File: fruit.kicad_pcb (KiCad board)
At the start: 2 copper layers, 161.6 x 100 mm, 178 parts, among them J1 PCB_Edge_PCI_Express_x4_Salmo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, J2 2086581051, J3 TSM-102-01-L-SV, J4 TSM-102-01-L-SV, J5 MEM2067-02-180-00-A_REVB, J6 USB4110-GF-A, J7 USB4110-GF-A, J8 1-2199119-6, U1 INA260, U10 LM3525M-H_NPOB, U11 USB3740B-AI2, U12 AP22653FDZ-7, U13 AP64501SP-13, U14 AP64501SP-13, U2 PCA9671BS,118, U3 PCA9671BS,118, U4 AP22653FDZ-7, U5 TPD8S009DSMR, U6 INA260, U7 MCP9808T-E_MC, U8 ADS7142IRUGR, U9 MCP9808T-E_MC

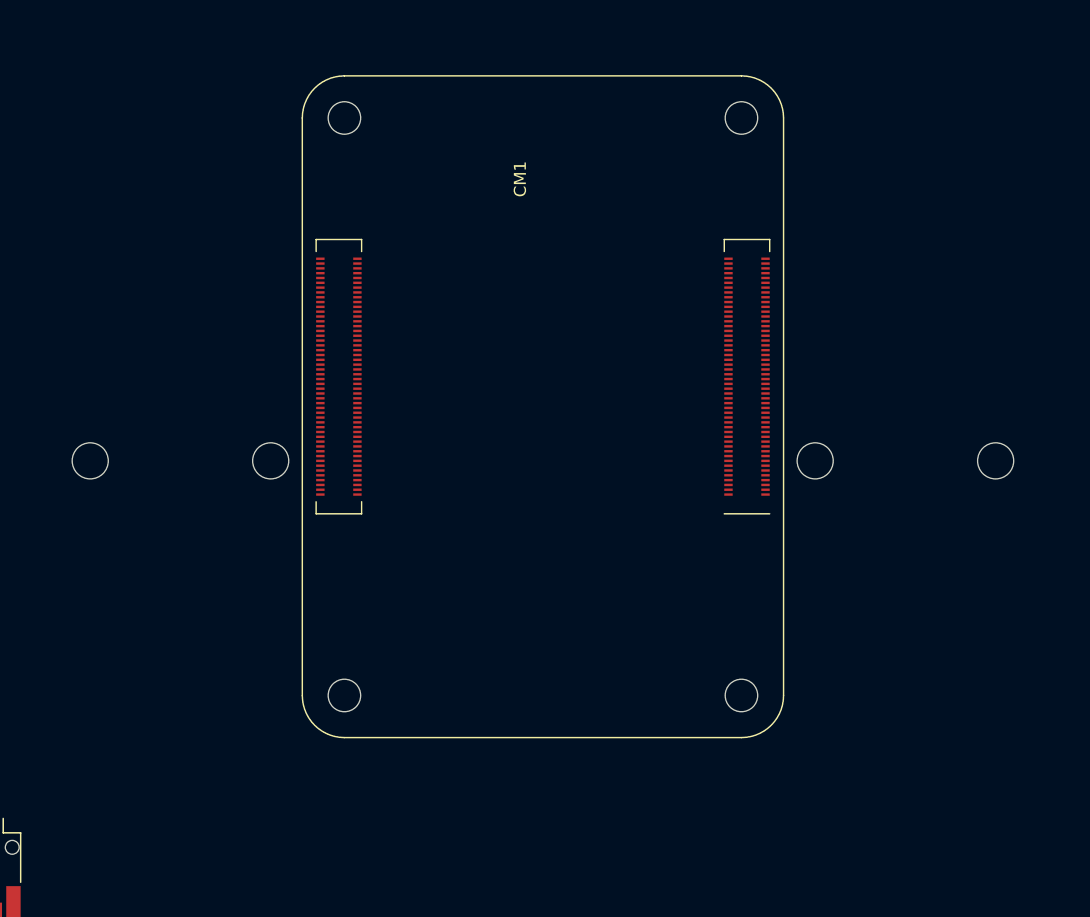
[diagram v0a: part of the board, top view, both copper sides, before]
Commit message: respin
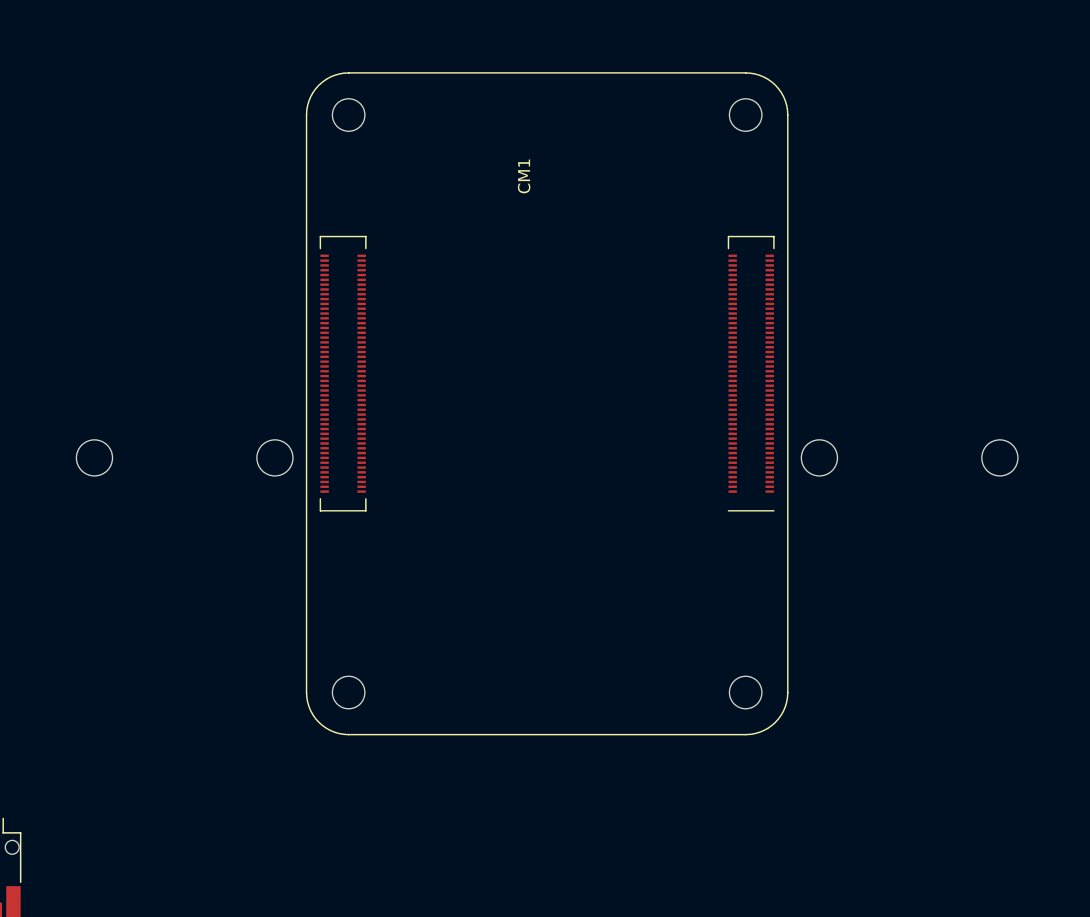
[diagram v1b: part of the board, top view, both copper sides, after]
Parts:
- moved CM1 0.43 mm to (121.4, 22.6)
- moved COOLER1 0.43 mm to (104.9, 51.1)
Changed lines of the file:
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@@
   )
   (footprint "Connector_RaspberryPi:Raspberry-Pi-4-Compute-Module_outline" (layer "F.Cu")
-    (at 121.05 22.86 180)
+    (at 121.402 22.614 180)
     (descr "Raspberry Pi 4 Compute Module")
     (tags "Raspberry Pi 4 Compute Module")
@@
   )
   (footprint "Mechanical_CoolingBlock:53-61mm_NorthBridge_45deg_arms" (layer "F.Cu")
-    (at 104.55 51.3 90)
+    (at 104.902 51.054 90)
     (descr "53-61mm mounting hole pattern and NorthBridge, 45 deg offset, and arms -- combined.")
     (property "Sheetfile" "fruit.kicad_sch")

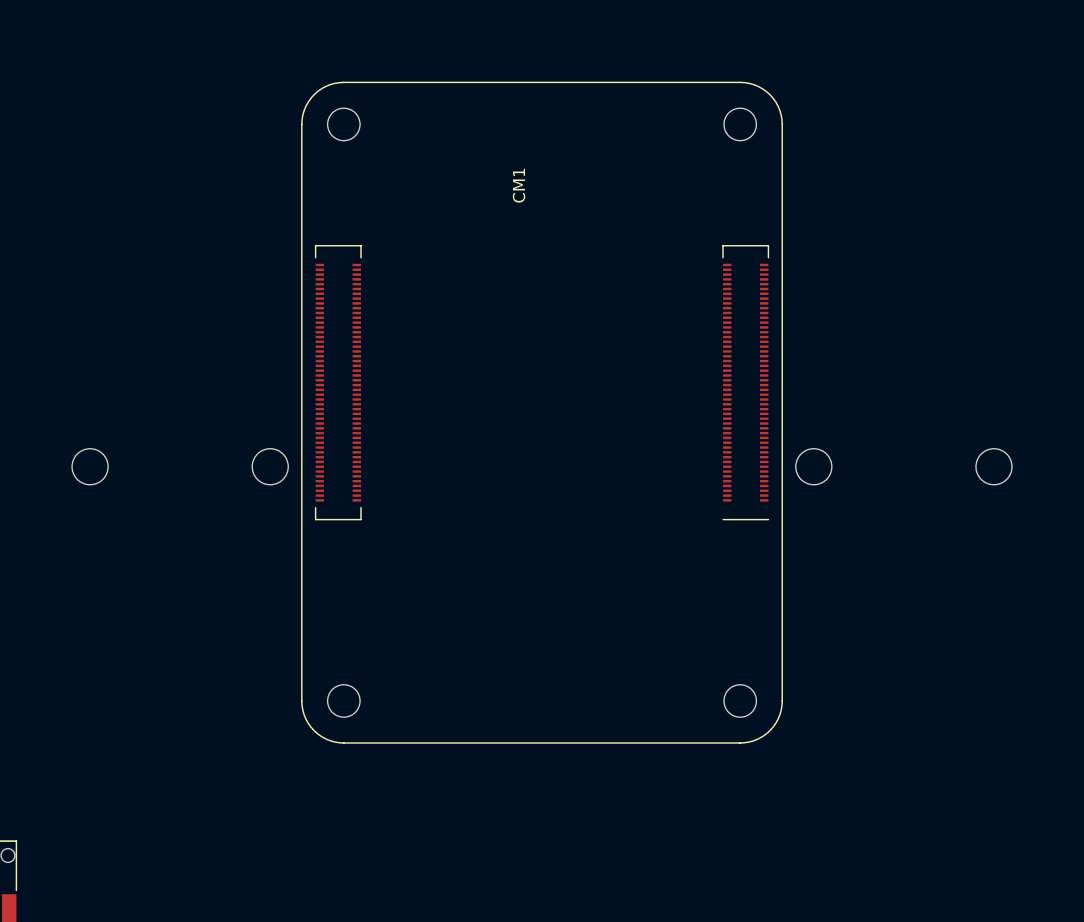
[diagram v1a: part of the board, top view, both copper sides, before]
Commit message: respin
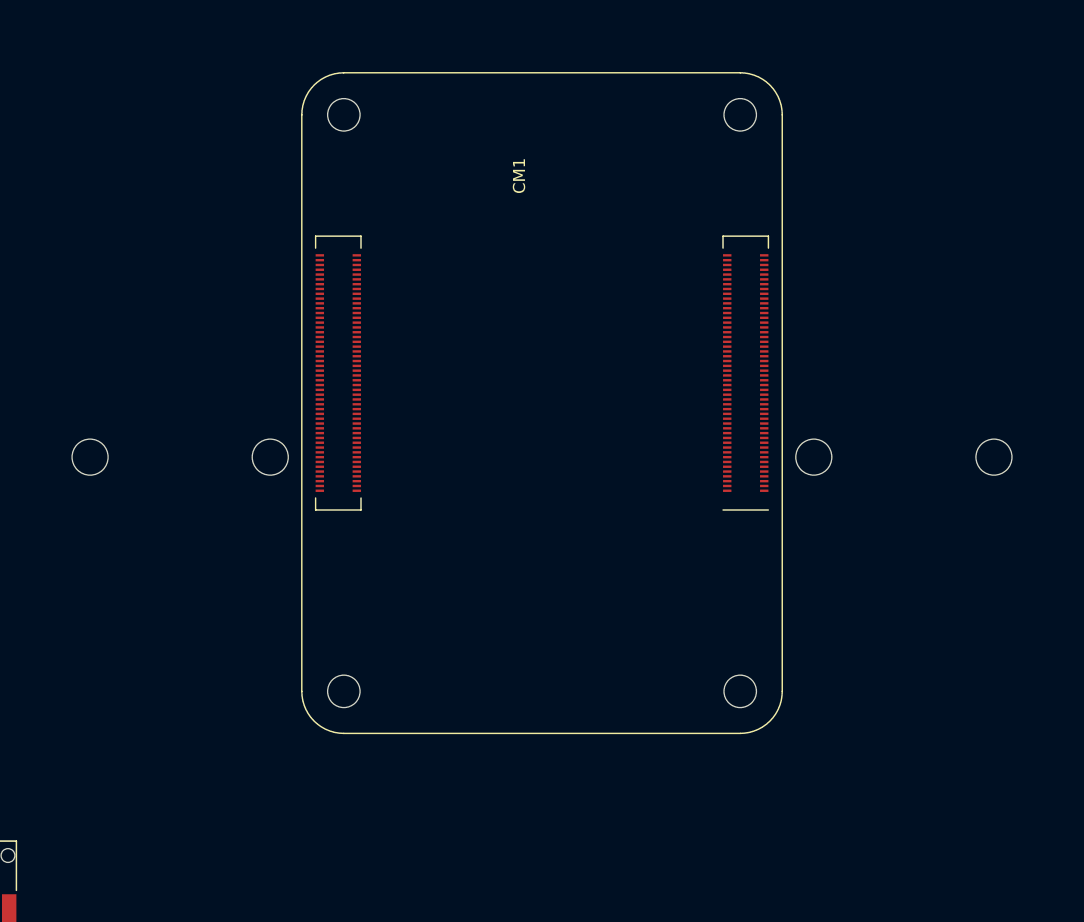
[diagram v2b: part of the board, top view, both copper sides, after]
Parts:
- moved COOLER1 0.80 mm to (104.9, 50.3)
- moved CM1 0.80 mm to (121.4, 21.8)
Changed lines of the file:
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@@
   )
   (footprint "Connector_RaspberryPi:Raspberry-Pi-4-Compute-Module_outline" (layer "F.Cu")
-    (at 121.402 22.614 180)
+    (at 121.402 21.814 180)
     (descr "Raspberry Pi 4 Compute Module")
     (tags "Raspberry Pi 4 Compute Module")
@@
   )
   (footprint "Mechanical_CoolingBlock:53-61mm_NorthBridge_45deg_arms" (layer "F.Cu")
-    (at 104.902 51.054 90)
+    (at 104.902 50.254 90)
     (descr "53-61mm mounting hole pattern and NorthBridge, 45 deg offset, and arms -- combined.")
     (property "Sheetfile" "fruit.kicad_sch")

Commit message: cosmetic
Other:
- board text added: "Place most components on this side"
- board text removed: "Place most components on this side."
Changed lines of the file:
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@@
     (effects (font (size 1 1) (thickness 0.15)))
   )
-  (gr_text "Place most components on this side." (at 80 -10) (layer "Cmts.User")
+  (gr_text "Place most components on this side" (at 80 -10) (layer "Cmts.User")
     (effects (font (size 3 3) (thickness 0.25)))
   )
